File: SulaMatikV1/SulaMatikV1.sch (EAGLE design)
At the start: 43 parts, among them IC1 REG1117, Q1 2N3904, Q2 2N5551, Q3 2N5551

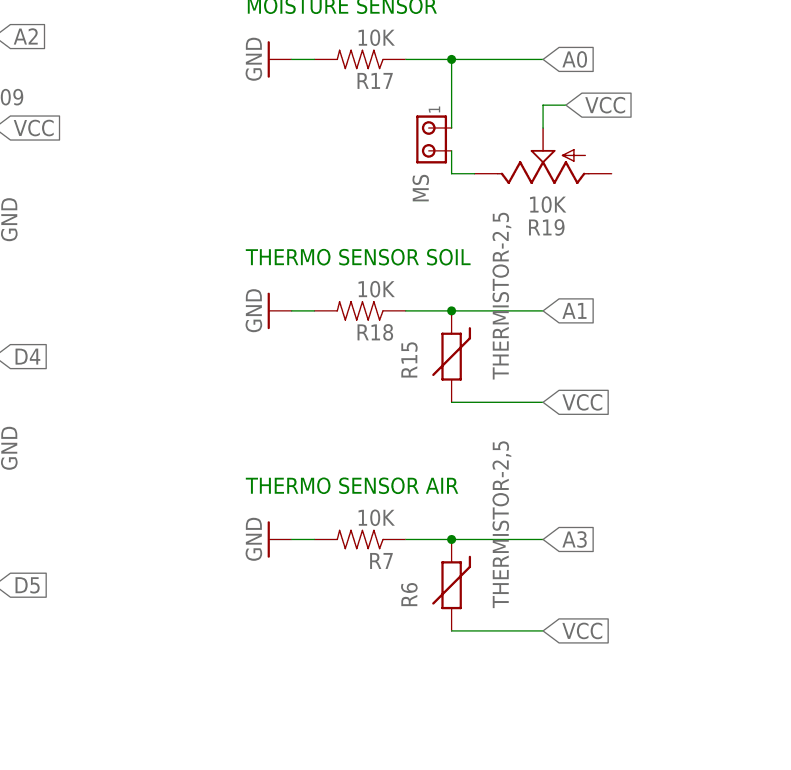
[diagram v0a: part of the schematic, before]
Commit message: v1
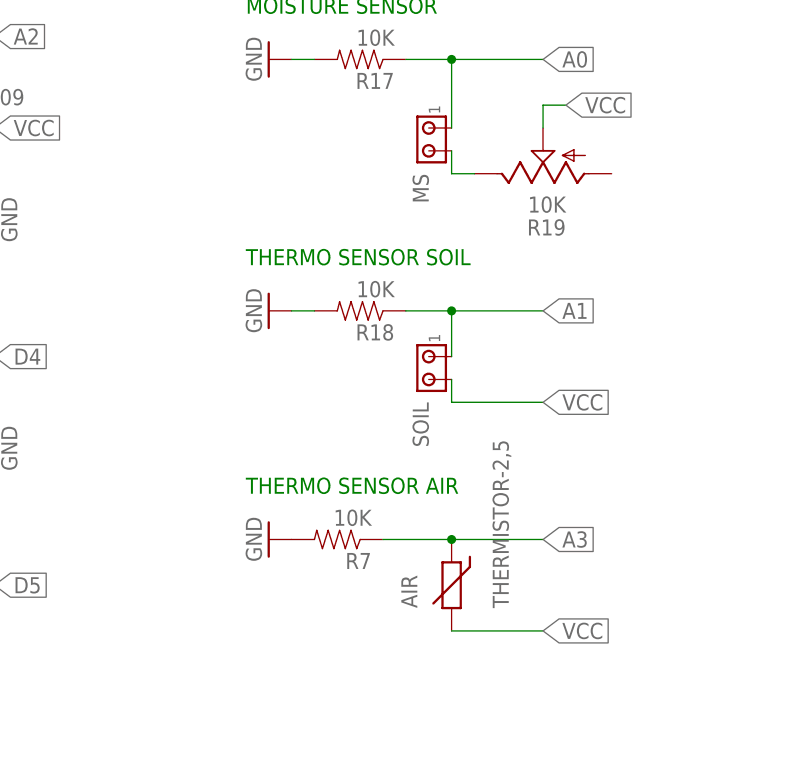
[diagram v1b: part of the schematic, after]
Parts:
- removed R15: THERMISTOR-2,5, varistor:THERMISTOR-2,5
- added SOIL: (no value), con-amp:MTA02-100
- LIGHT, MS, PUMP, PW: device con-amp:MTA02-156 -> con-amp:MTA02-100
- renumbered R6 to AIR
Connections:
- net A1: now also SOIL.1; no longer R15.1
- net A3: now also R7.1
- net VCC: now also SOIL.2; no longer R15.2
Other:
- moved on the sheet: R7
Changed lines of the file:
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@@
 <part name="JP7" library="SparkFun" deviceset="M12" device="PTH" value=""/>
 <part name="JP2" library="SparkFun" deviceset="M02" device="PTH"/>
-<part name="PUMP" library="con-amp" deviceset="MTA02-156" device=""/>
+<part name="PUMP" library="con-amp" deviceset="MTA02-100" device=""/>
 <part name="Q3" library="semicon-smd-ipc" deviceset="NPN-TRANSISTOR_" device="SOT23" value="2N5551"/>
 <part name="R11" library="SparkFun-Passives" deviceset="RESISTOR" device="0805-RES" value="1K"/>
@@
 <part name="R12" library="SparkFun-Passives" deviceset="RESISTOR" device="0805-RES" value="330"/>
 <part name="F1" library="_hhn_PtcFuses_Siba_r500_Ozan" deviceset="SIBA194600*" device="" value="1.5A"/>
-<part name="PW" library="con-amp" deviceset="MTA02-156" device=""/>
+<part name="PW" library="con-amp" deviceset="MTA02-100" device=""/>
 <part name="R13" library="SparkFun-Passives" deviceset="RESISTOR" device="0805-RES" value="10k"/>
 <part name="GND3" library="supply1" deviceset="GND" device=""/>
 <part name="IC1" library="burr-brown" deviceset="REG1117" device=""/>
-<part name="LIGHT" library="con-amp" deviceset="MTA02-156" device=""/>
+<part name="LIGHT" library="con-amp" deviceset="MTA02-100" device=""/>
 <part name="Q1" library="semicon-smd-ipc" deviceset="NPN-TRANSISTOR_" device="SOT23" value="2N3904"/>
 <part name="R14" library="SparkFun-Passives" deviceset="RESISTOR" device="0805-RES" value="1K"/>
 <part name="D3" library="SparkFun-DiscreteSemi" deviceset="DIODE" device="SMA"/>
 <part name="GND4" library="supply1" deviceset="GND" device=""/>
-<part name="R15" library="varistor" deviceset="THERMISTOR" device="-2,5"/>
 <part name="PH1" library="photo-elements" deviceset="A10" device="" technology="50_09"/>
 <part name="GND6" library="supply1" deviceset="GND" device=""/>
@@
 <part name="GND8" library="supply1" deviceset="GND" device=""/>
 <part name="R18" library="SparkFun-Passives" deviceset="RESISTOR" device="0805-RES" value="10K"/>
-<part name="MS" library="con-amp" deviceset="MTA02-156" device=""/>
+<part name="MS" library="con-amp" deviceset="MTA02-100" device=""/>
 <part name="R19" library="pot" deviceset="TRIM_US-" device="CA6V" value="10K"/>
 <part name="SV2" library="con-lsta" deviceset="FE08-1" device=""/>
@@
 <part name="R5" library="SparkFun-Passives" deviceset="RESISTOR" device="0805-RES" value="10k"/>
 <part name="GND11" library="supply1" deviceset="GND" device=""/>
-<part name="R6" library="varistor" deviceset="THERMISTOR" device="-2,5"/>
+<part name="AIR" library="varistor" deviceset="THERMISTOR" device="-2,5"/>
 <part name="GND12" library="supply1" deviceset="GND" device=""/>
 <part name="R7" library="SparkFun-Passives" deviceset="RESISTOR" device="0805-RES" value="10K"/>
 <part name="SV1" library="con-lstb" deviceset="MA04-1" device=""/>
+<part name="SOIL" library="con-amp" deviceset="MTA02-100" device=""/>
 </parts>
 <sheets>
@@
 <instance part="D3" gate="G$1" x="162.56" y="129.54"/>
 <instance part="GND4" gate="1" x="172.72" y="121.92" rot="R90"/>
-<instance part="R15" gate="G$1" x="210.82" y="78.74" rot="R90"/>
 <instance part="PH1" gate="G$1" x="149.86" y="109.22"/>
 <instance part="GND6" gate="1" x="129.54" y="114.3" rot="R270"/>
@@
 <instance part="R5" gate="G$1" x="137.16" y="60.96" rot="R270"/>
 <instance part="GND11" gate="1" x="160.02" y="68.58" rot="R90"/>
-<instance part="R6" gate="G$1" x="210.82" y="53.34" rot="R90"/>
+<instance part="AIR" gate="G$1" x="210.82" y="53.34" rot="R90"/>
 <instance part="GND12" gate="1" x="190.5" y="58.42" rot="R270"/>
-<instance part="R7" gate="G$1" x="200.66" y="58.42" rot="R180"/>
+<instance part="R7" gate="G$1" x="198.12" y="58.42" rot="R180"/>
 <instance part="SV1" gate="1" x="96.52" y="27.94"/>
+<instance part="SOIL" gate="G$1" x="208.28" y="78.74" rot="MR270"/>
 </instances>
 <busses>
@@
 <pinref part="R7" gate="G$1" pin="2"/>
 <pinref part="GND12" gate="1" pin="GND"/>
-<wire x1="193.04" y1="58.42" x2="195.58" y2="58.42" width="0.1524" layer="91"/>
 </segment>
 </net>
@@
 <wire x1="210.82" y1="73.66" x2="220.98" y2="73.66" width="0.1524" layer="91"/>
 <label x="220.98" y="73.66" size="1.778" layer="95" xref="yes"/>
-<pinref part="R15" gate="G$1" pin="2"/>
+<pinref part="SOIL" gate="G$1" pin="2"/>
+<wire x1="210.82" y1="73.66" x2="210.82" y2="76.2" width="0.1524" layer="91"/>
 </segment>
 <segment>
@@
 <wire x1="210.82" y1="48.26" x2="220.98" y2="48.26" width="0.1524" layer="91"/>
 <label x="220.98" y="48.26" size="1.778" layer="95" xref="yes"/>
-<pinref part="R6" gate="G$1" pin="2"/>
+<pinref part="AIR" gate="G$1" pin="2"/>
 </segment>
 </net>
@@
 <segment>
 <label x="220.98" y="58.42" size="1.778" layer="95" xref="yes"/>
-<wire x1="205.74" y1="58.42" x2="210.82" y2="58.42" width="0.1524" layer="91"/>
-<pinref part="R6" gate="G$1" pin="1"/>
+<wire x1="203.2" y1="58.42" x2="210.82" y2="58.42" width="0.1524" layer="91"/>
+<pinref part="AIR" gate="G$1" pin="1"/>
 <junction x="210.82" y="58.42"/>
 <wire x1="210.82" y1="58.42" x2="220.98" y2="58.42" width="0.1524" layer="91"/>
+<pinref part="R7" gate="G$1" pin="1"/>
 </segment>
 </net>
@@
 <segment>
 <label x="220.98" y="83.82" size="1.778" layer="95" xref="yes"/>
+<pinref part="R18" gate="G$1" pin="1"/>
 <wire x1="205.74" y1="83.82" x2="210.82" y2="83.82" width="0.1524" layer="91"/>
-<pinref part="R18" gate="G$1" pin="1"/>
-<pinref part="R15" gate="G$1" pin="1"/>
+<pinref part="SOIL" gate="G$1" pin="1"/>
 <wire x1="210.82" y1="83.82" x2="220.98" y2="83.82" width="0.1524" layer="91"/>
+<wire x1="210.82" y1="78.74" x2="210.82" y2="83.82" width="0.1524" layer="91"/>
 <junction x="210.82" y="83.82"/>
 </segment>
